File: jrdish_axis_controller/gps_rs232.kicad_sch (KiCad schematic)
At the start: 17 parts, among them CN10 KF2EDGR-2.54-2P, CN11 KF2EDGR-2.54-3P, Q3 2N7002, U8 SP3232EEY-L/TR

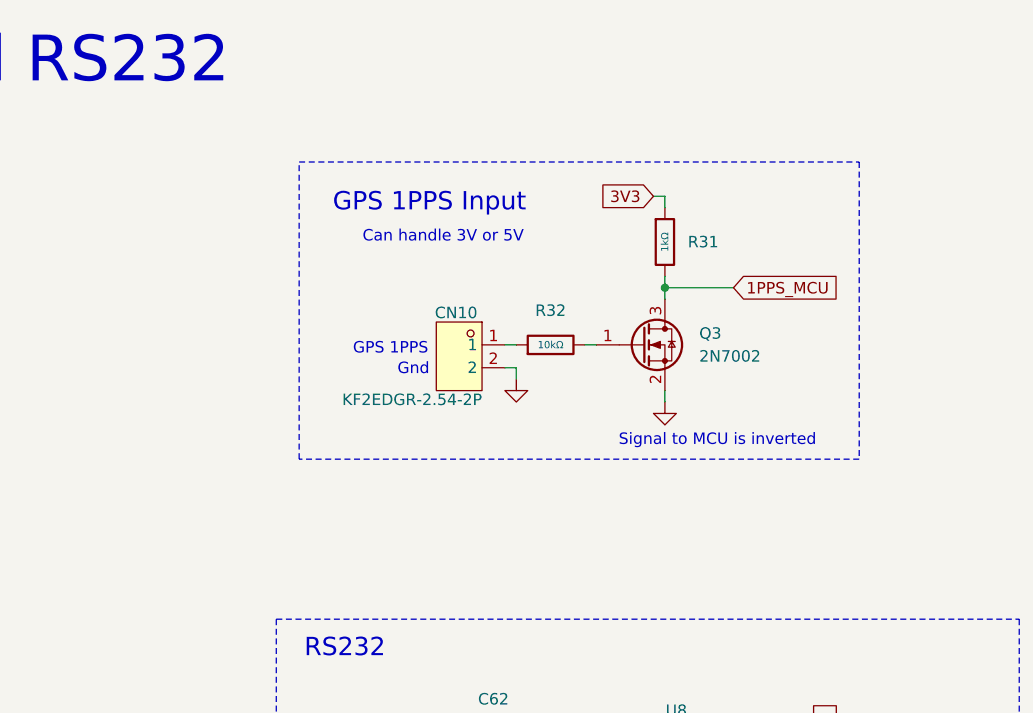
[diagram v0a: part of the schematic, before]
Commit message: Making refinements
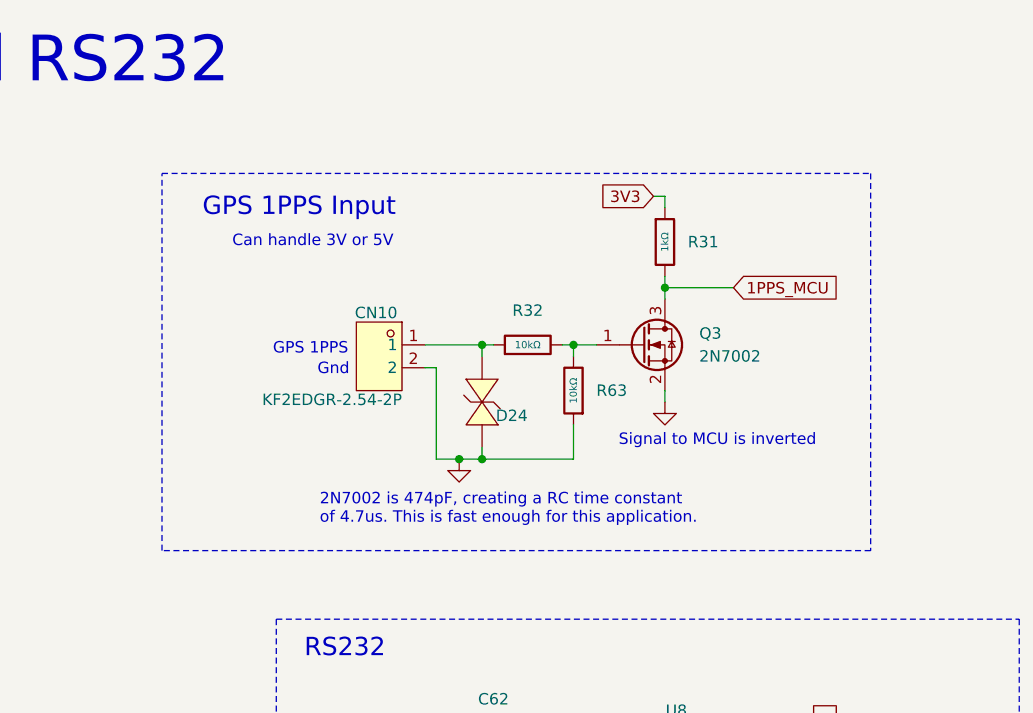
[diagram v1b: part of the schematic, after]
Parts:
- added D24: TPESD0402G05V, MyParts:D0402-BI, symbol MyParts:TPESD0402G05V
- added R63: 10kΩ, PCM_JLCPCB:R_0402, symbol PCM_JLCPCB-Resistors:0402,10kΩ
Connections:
- net GND: now also D24.2 (A), R63.1
- net at CN10.1, R32.1: now also D24.1 (K)
- net at Q3.1 (G), R32.2: now also R63.2
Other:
- note added: "2N7002 is 474pF, creating a RC time constant of 4.7us. This is fast enough for this application."
- moved on the sheet: CN10, R32
